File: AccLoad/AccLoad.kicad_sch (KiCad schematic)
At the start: 8 parts

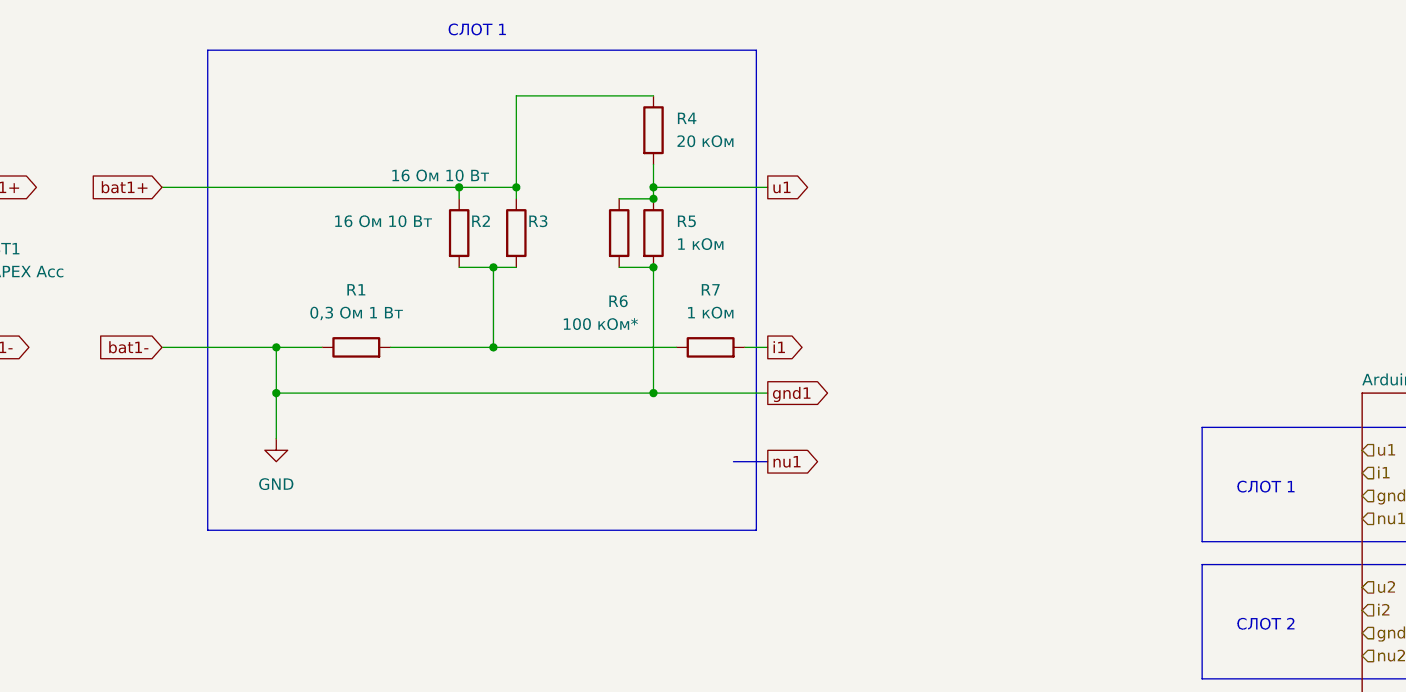
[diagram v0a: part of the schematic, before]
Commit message: star PCB designing
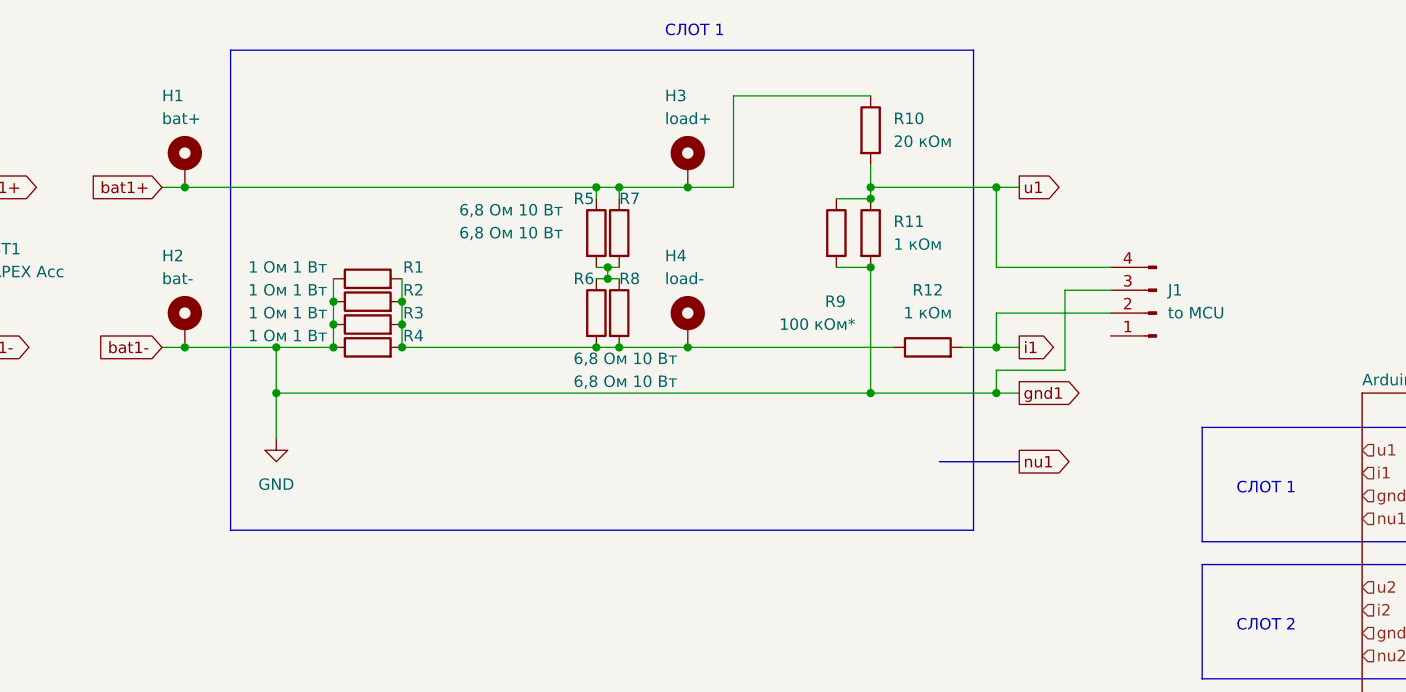
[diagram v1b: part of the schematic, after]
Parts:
- added H1: bat+, MountingHole:MountingHole_2.2mm_M2_DIN965_Pad_TopBottom, symbol Mechanical:MountingHole_Pad
- added H2: bat-, MountingHole:MountingHole_2.2mm_M2_DIN965_Pad_TopBottom, symbol Mechanical:MountingHole_Pad
- added H3: load+, MountingHole:MountingHole_2.2mm_M2_DIN965_Pad_TopBottom, symbol Mechanical:MountingHole_Pad
- added H4: load-, MountingHole:MountingHole_2.2mm_M2_DIN965_Pad_TopBottom, symbol Mechanical:MountingHole_Pad
- added J1: to MCU, Connector_JST:JST_EH_B4B-EH-A_1x04_P2.50mm_Vertical, symbol Connector:Conn_01x04_Male
- added R1, R2: 1 Ом 1 Вт, Resistor_SMD:R_2512_6332Metric_Pad1.40x3.35mm_HandSolder, symbol Device:R
- added R6, R7, R8: 6,8 Ом 10 Вт, symbol Device:R
- BT1: now left out of the parts list
- R10: renamed from R4; footprint (none) -> Resistor_SMD:R_0805_2012Metric_Pad1.20x1.40mm_HandSolder
- R11: renamed from R5; footprint (none) -> Resistor_SMD:R_0805_2012Metric_Pad1.20x1.40mm_HandSolder
- R12: renamed from R7; footprint (none) -> Resistor_SMD:R_0805_2012Metric_Pad1.20x1.40mm_HandSolder
- R3: value 16 Ом 10 Вт -> 1 Ом 1 Вт; footprint (none) -> Resistor_SMD:R_2512_6332Metric_Pad1.40x3.35mm_HandSolder
- R4: renamed from R1; value 0,3 Ом 1 Вт -> 1 Ом 1 Вт; footprint (none) -> Resistor_SMD:R_2512_6332Metric_Pad1.40x3.35mm_HandSolder
- R5: renamed from R2; value 16 Ом 10 Вт -> 6,8 Ом 10 Вт; now left out of the parts list
- R9: renamed from R6; footprint (none) -> Resistor_SMD:R_0805_2012Metric_Pad1.20x1.40mm_HandSolder
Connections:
- net GND: now also R3.1, H2.1, J1.3 (Pin_3), R1.1, R2.1
- net bat1+: now also H1.1, H3.1, R7.1; no longer R3.1
- net i1: now also J1.2 (Pin_2)
- net u1: now also J1.4 (Pin_4)
- net at R12.1, R3.2, R4.2: now also H4.1, R1.2, R2.2, R6.2, R8.2; no longer R5.2
- new net: R5.2, R6.1, R7.2, R8.1
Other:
- moved on the sheet: R10, R11, R12, R4, R5, R9
